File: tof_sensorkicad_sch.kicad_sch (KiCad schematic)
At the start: 17 parts

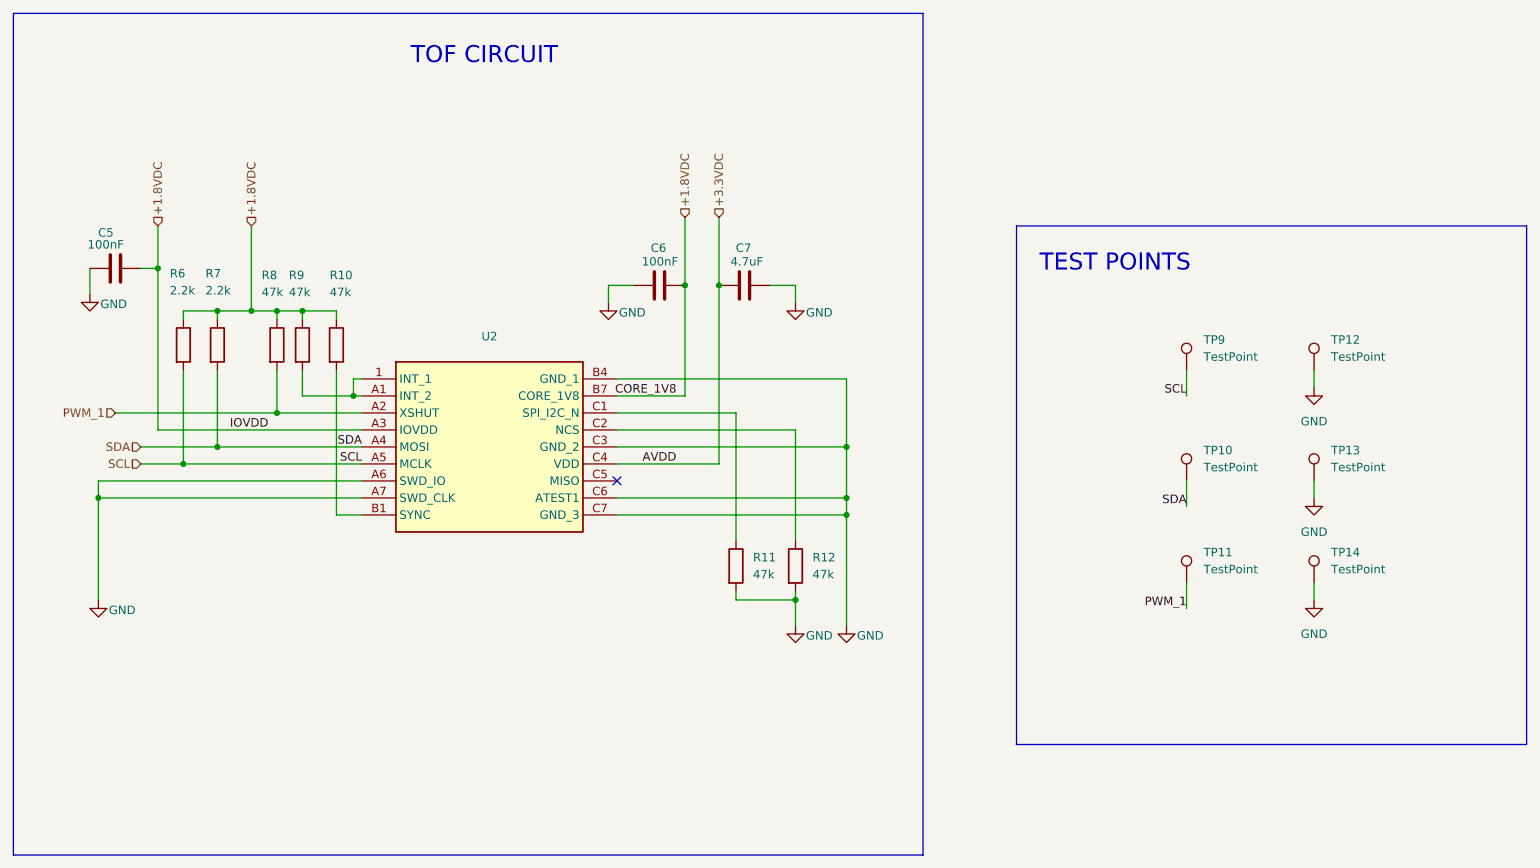
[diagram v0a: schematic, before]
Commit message: latest updates, up to v2
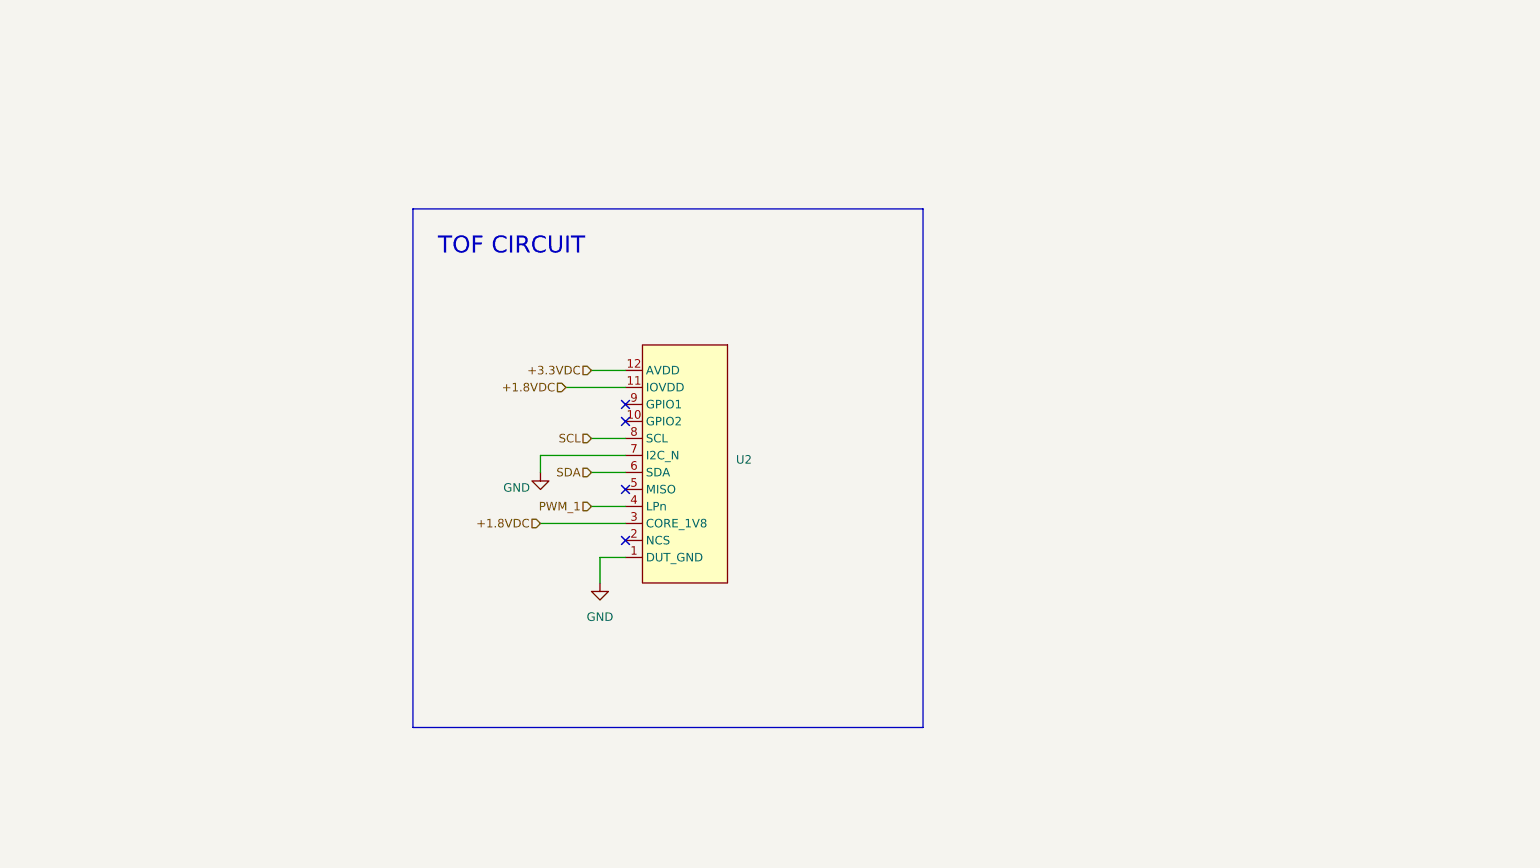
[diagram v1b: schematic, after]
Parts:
- removed C5, C6: 100nF, Capacitor_SMD:C_0805_2012Metric_Pad1.18x1.45mm_HandSolder, symbol Device:C
- removed C7: 4.7uF, Capacitor_SMD:C_0805_2012Metric_Pad1.18x1.45mm_HandSolder, symbol Device:C
- removed R10, R11, R12, R8, R9: 47k, Resistor_SMD:R_0805_2012Metric_Pad1.20x1.40mm_HandSolder, symbol Device:R
- removed R6, R7: 2.2k, Resistor_SMD:R_0805_2012Metric_Pad1.20x1.40mm_HandSolder, symbol Device:R
- removed TP10, TP11, TP12, TP13, TP14, TP9: TestPoint, TestPoint:TestPoint_Pad_D2.0mm, symbol Connector:TestPoint
- U2: footprint VL53L8CXV0GC1 -> 00_parts_lib:SATEL-VL53L8A; symbol 00_project_parts:VL53L8CXV0GC_1 -> 00_project_parts:SATEL-VL53L8A; Height 1.8 -> (none); Manufacturer_Name STMicroelectronics -> (none); Manufacturer_Part_Number VL53L8CXV0GC/1 -> (none); Mouser Part Number 511-VL53L8CXV0GC/1 -> (none); Mouser Price/Stock https://www.mouser.co.uk/ProductDetail/STMicroelectronics/V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 -> (none)
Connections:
- net +1.8VDC: now also U2.11 (IOVDD), U2.3 (CORE_1V8); no longer U2.A3 (IOVDD), U2.B7 (CORE_1V8)
- net +3.3VDC: now also U2.12 (AVDD); no longer U2.C4 (VDD)
- net GND: now also U2.1 (DUT_GND), U2.7 (I2C_N); no longer U2.A6 (SWD_IO), U2.A7 (SWD_CLK), U2.B4 (GND_1), U2.C3 (GND_2), U2.C6 (ATEST1), U2.C7 (GND_3)
- net PWM_1: now also U2.4 (LPn); no longer U2.A2 (XSHUT)
- net SCL: now also U2.8 (SCL); no longer U2.A5 (MCLK)
- net SDA: now also U2.6 (SDA); no longer U2.A4 (MOSI)
- no-connect marks 1 -> 4
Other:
- note removed: "TEST POINTS"
